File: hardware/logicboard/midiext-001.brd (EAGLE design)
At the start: 72 x 72 mm, 29 parts, among them IC1 74ALS05N, IC2 LTC485N, IC3 LTC485N, J1 PWR, J2 MIDIOUT, J3 MIDIIN, J4 LED, J5 MIDIRX, J6 MIDITX, J7 LED

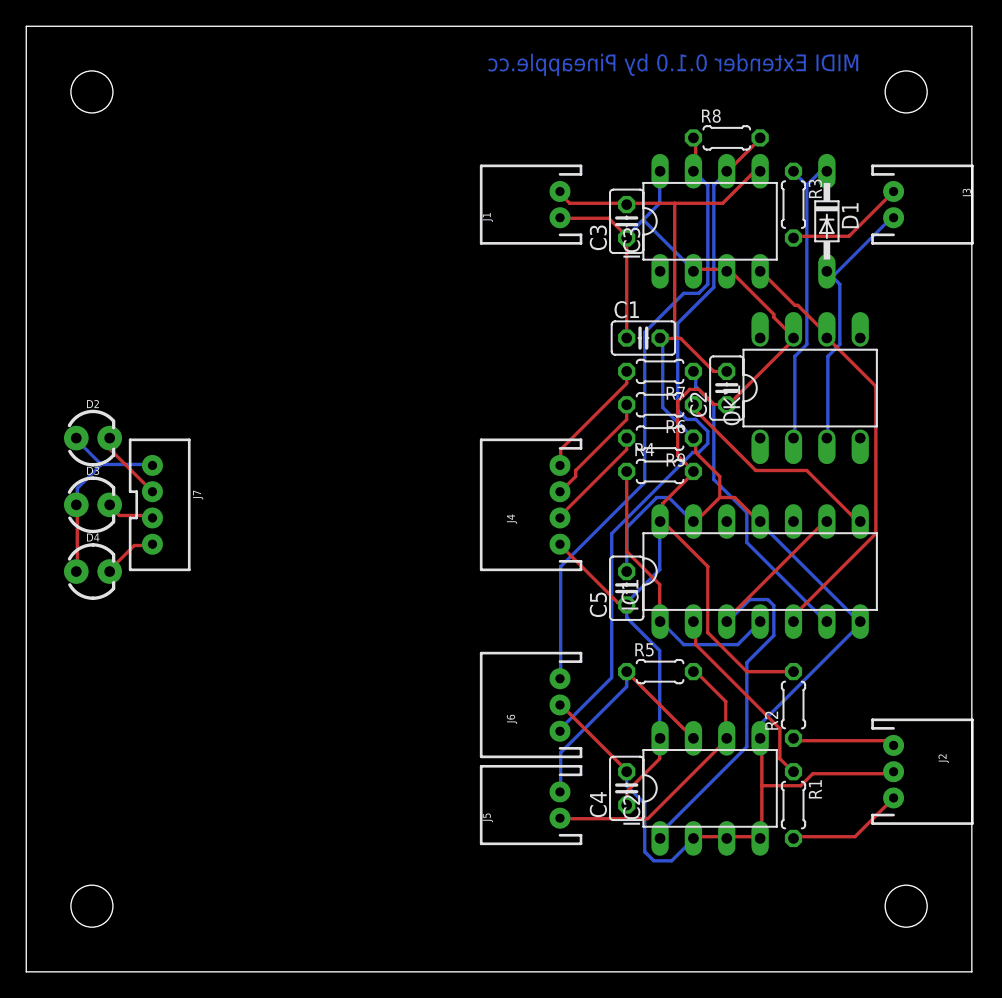
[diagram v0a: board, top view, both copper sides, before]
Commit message: Second try.
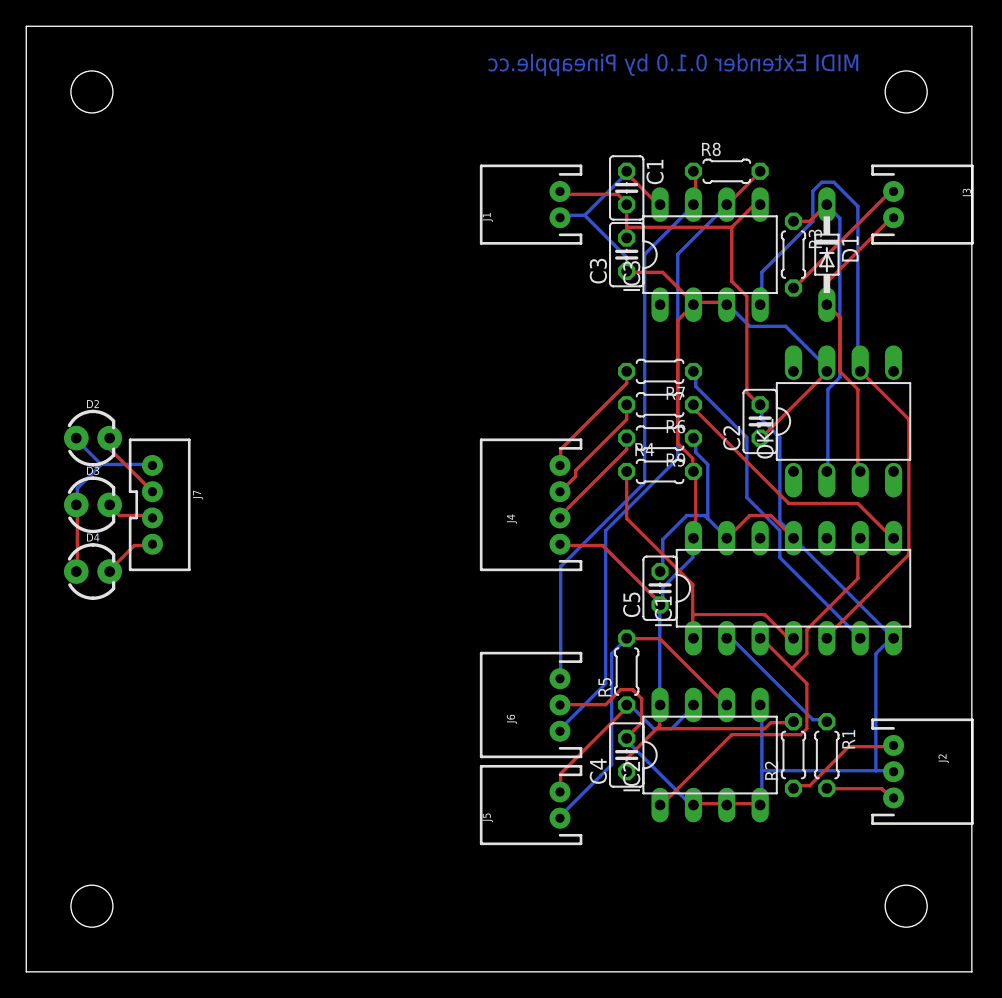
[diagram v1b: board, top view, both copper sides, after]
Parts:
- moved C1 11.5 mm to (45.7, 59.7), turned to 270 degrees
- moved R1 4.58 mm to (61.0, 16.5)
- moved R3 3.81 mm to (58.4, 54.6)
- moved R2 3.81 mm to (58.4, 16.5)
- moved C2 3.59 mm to (55.9, 41.9)
- moved OK1 3.59 mm to (62.2, 41.9)
- moved IC1 2.84 mm to (58.4, 29.2)
- moved C4 2.54 mm to (45.7, 16.5)
- moved IC2 2.54 mm to (52.1, 16.5)
- moved C3 2.54 mm to (45.7, 54.6)
- moved C5 2.54 mm to (48.3, 29.2)
- moved D1 2.54 mm to (61.0, 54.6)
- moved IC3 2.54 mm to (52.1, 54.6)
- moved R5 2.54 mm to (45.7, 22.9), turned to 90 degrees
- moved R8 2.54 mm to (53.3, 61.0)
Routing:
- net COM2: track 33.2 -> 52.0 mm
- net VCC: track 107.5 -> 101.5 mm
- net TX+: track 54.0 -> 48.9 mm
- net N$2: track 14.6 -> 10.4 mm
- net TX-: track 47.2 -> 43.0 mm
- net RX+: track 21.5 -> 25.5 mm
- net MIDITX-: track 8.91 -> 5.37 mm
- net N$7: track 16.6 -> 19.6 mm
- net RX-: track 18.5 -> 15.5 mm
- net N$1: track 36.7 -> 34.1 mm
- net MIDIRX-: track 20.2 -> 22.6 mm
- net N$6: track 23.4 -> 25.7 mm
- net N$3: track 21.6 -> 23.2 mm
- net MIDIRX+: track 9.10 -> 10.7 mm
- net MIDITX+: track 7.86 -> 9.00 mm
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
